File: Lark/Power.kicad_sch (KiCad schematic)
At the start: 39 parts, among them J1 54-00128, Q1 SISS65DN-T1-GE3, Q2 MMBT2222A-7-F, U5 BD9E302EFJ-E2, U6 BD9G102G-LBTR, U7 LD39200PU33R

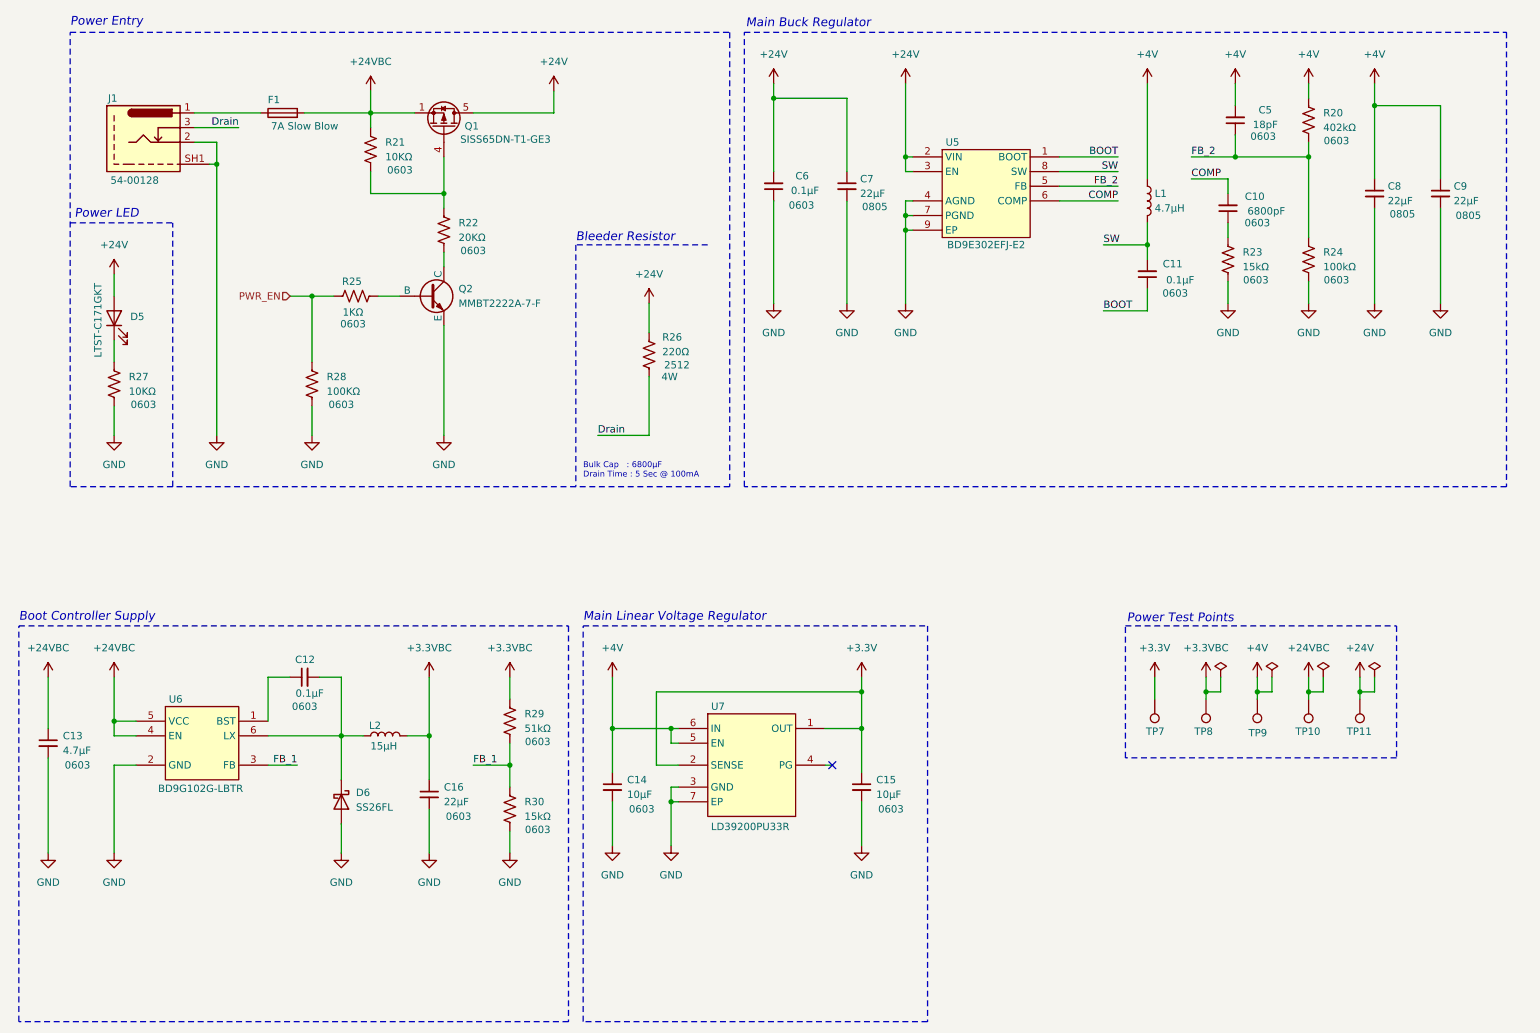
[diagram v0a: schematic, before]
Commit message: Update, WIP
- Added TVS diode to 24v Supply.
- Fixed bleeder circuit at some point (I think it was this commit)
- Added Jumper to connect NTC to ADC. (again I think it was this commit)
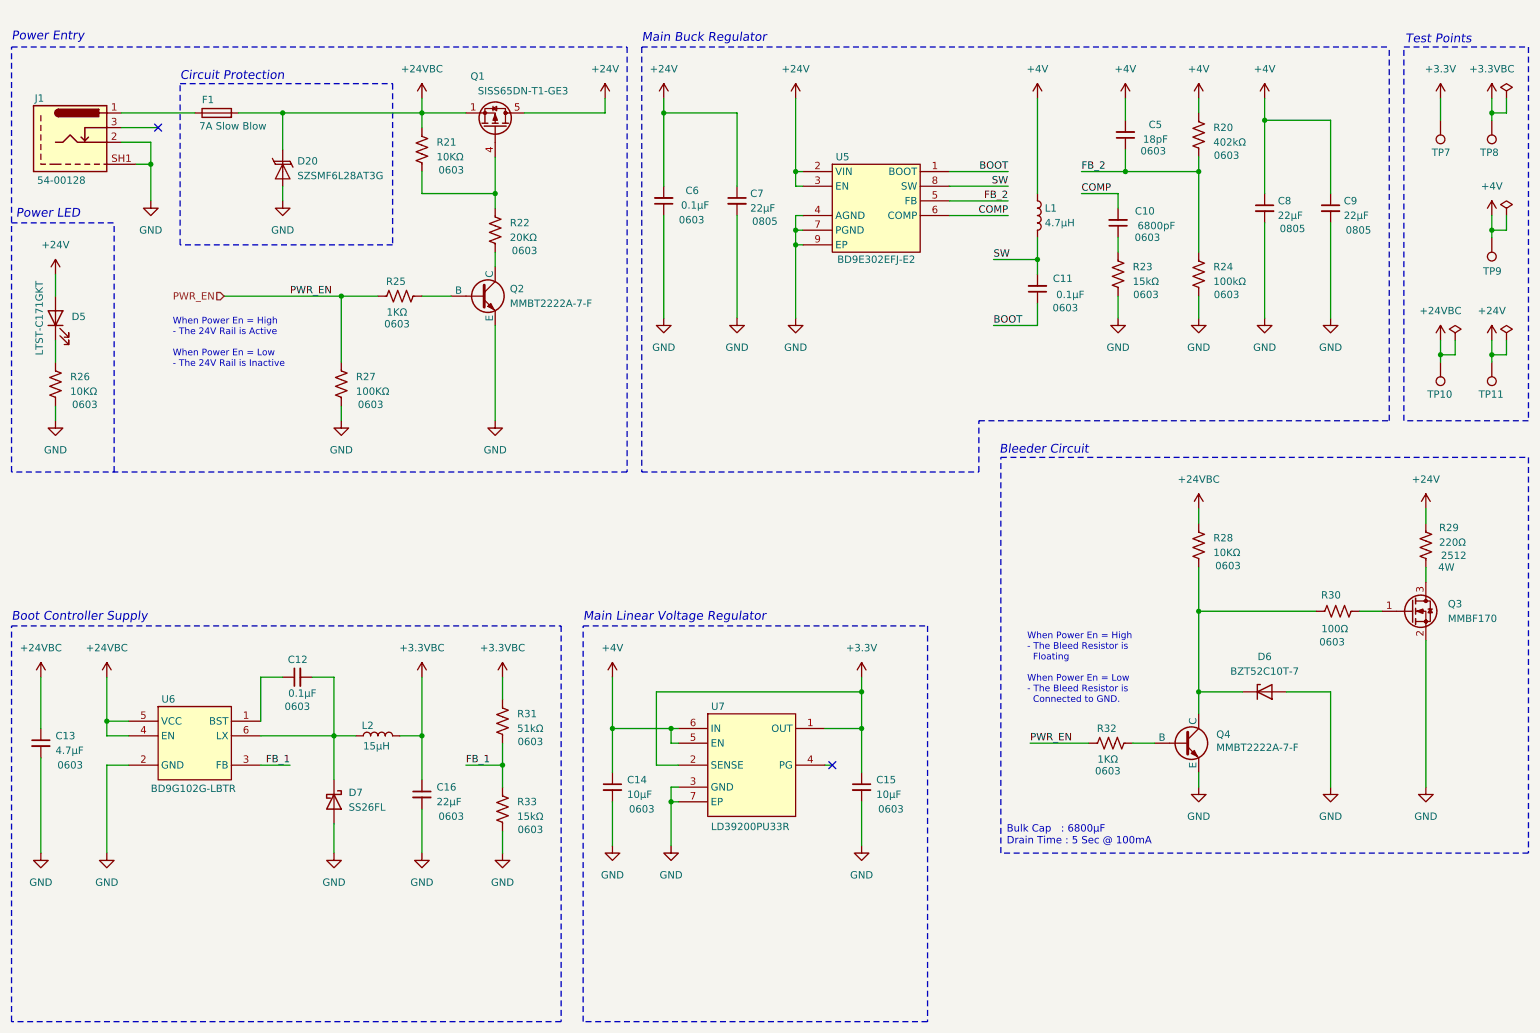
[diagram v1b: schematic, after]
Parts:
- added D20: SZSMF6L28AT3G, Littelfuse Inc:SZSMF6L28AT3G, symbol Littelfuse Inc:SZSMF6L28AT3G
- added D6: BZT52C10T-7, Diodes Incorporated:BZT52C10T-7, symbol Diodes Incorporated:BZT52C10T-7
- added Q3: MMBF170, onsemi:MMBF170, symbol onsemi:MMBF170
- added Q4: MMBT2222A-7-F, Diodes Incorporated:MMBT2222A-7-F, symbol Diodes Incorporated:MMBT2222A-7-F
- added R28: 10KΩ, Stackpole:R_0603, symbol Stackpole:Resistor
- added R30: 100Ω, Stackpole:R_0603, symbol Stackpole:Resistor
- added R32: 1KΩ, Stackpole:R_0603, symbol Stackpole:Resistor
- renumbered D6 to D7, R27 to R26, R28 to R27, R26 to R29, R29 to R31, R30 to R33
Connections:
- net +24VBC: now also D20.1 (Cathode), R28.1
- net GND: now also D20.2 (Anode), D6.2 (A), Q3.2 (S), Q4.2 (E)
- net PWR_EN: now also R32.1
- net Drain: no longer names the net of R29.2
- net Drain: now also Q3.3 (D); no longer J1.3
- new net: D6.1 (K), Q4.3 (C), R28.2, R30.1
- new net: Q4.1 (B), R32.2
- new net: Q3.1 (G), R30.2
- no-connect marks 1 -> 2
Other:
- note added: "Bleeder Circuit"
- note added: "Circuit Protection"
- note added: "Test Points"
- note added: "When Power En = High - The 24V Rail is Active When Power En = Low - The 24V Rail is Inactive"
- note added: "When Power En = High - The Bleed Resistor is Floating When Power En = Low - The Bleed Resistor is Connected to GND."
- note removed: "Bleeder Resistor"
- note removed: "Power Test Points"
- moved on the sheet: C10, C11, C12, C13, C16, C5, C6, C7, C8, C9, D5, D7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
